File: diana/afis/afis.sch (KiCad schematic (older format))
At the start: 88 parts

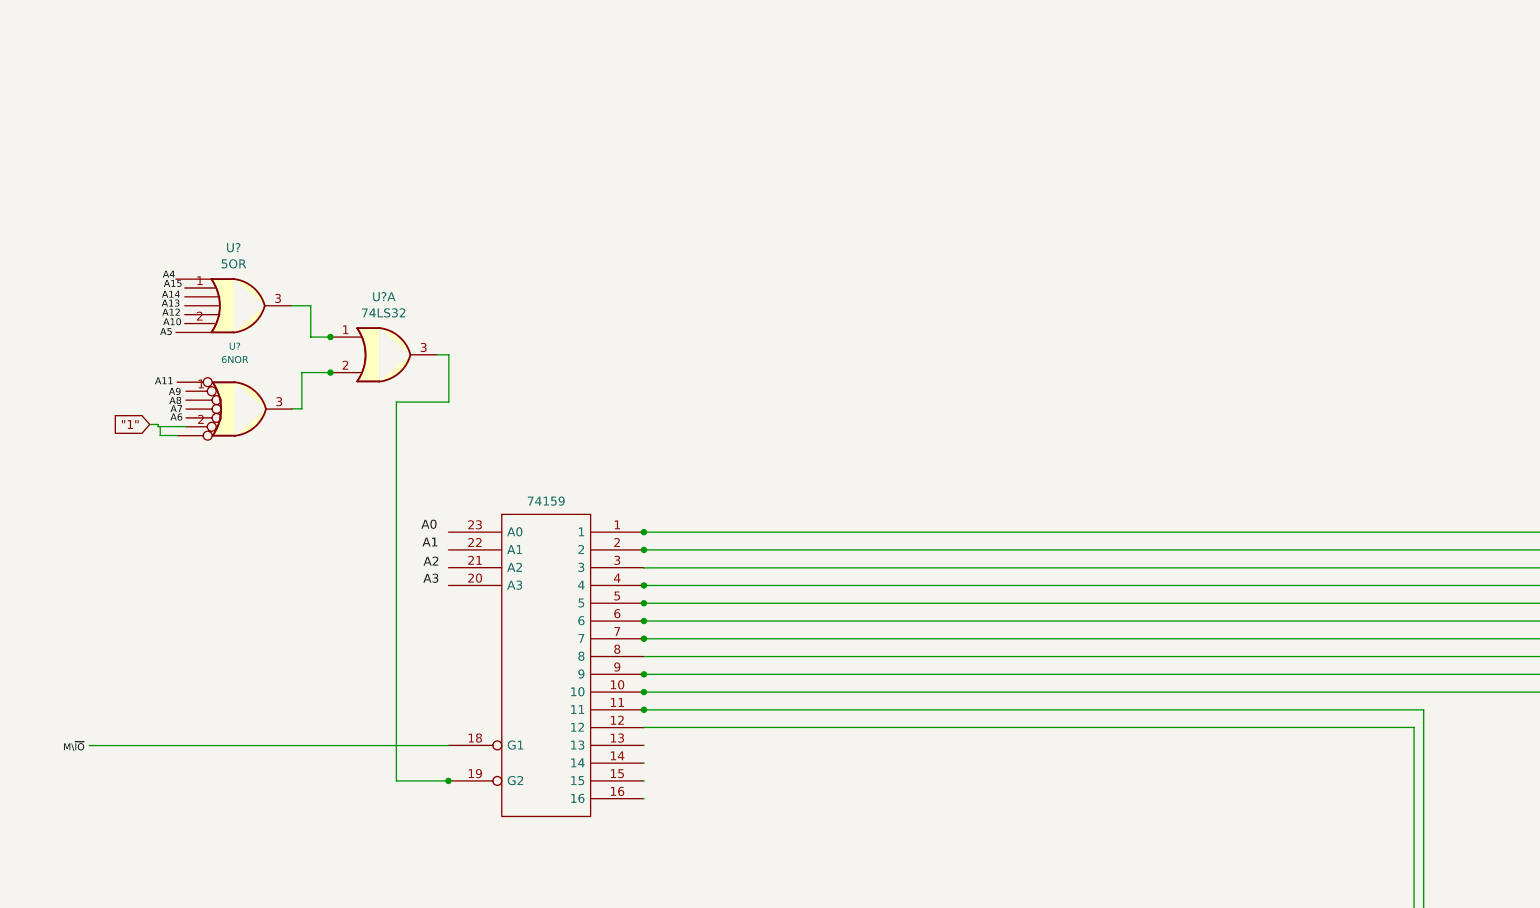
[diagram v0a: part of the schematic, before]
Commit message: c
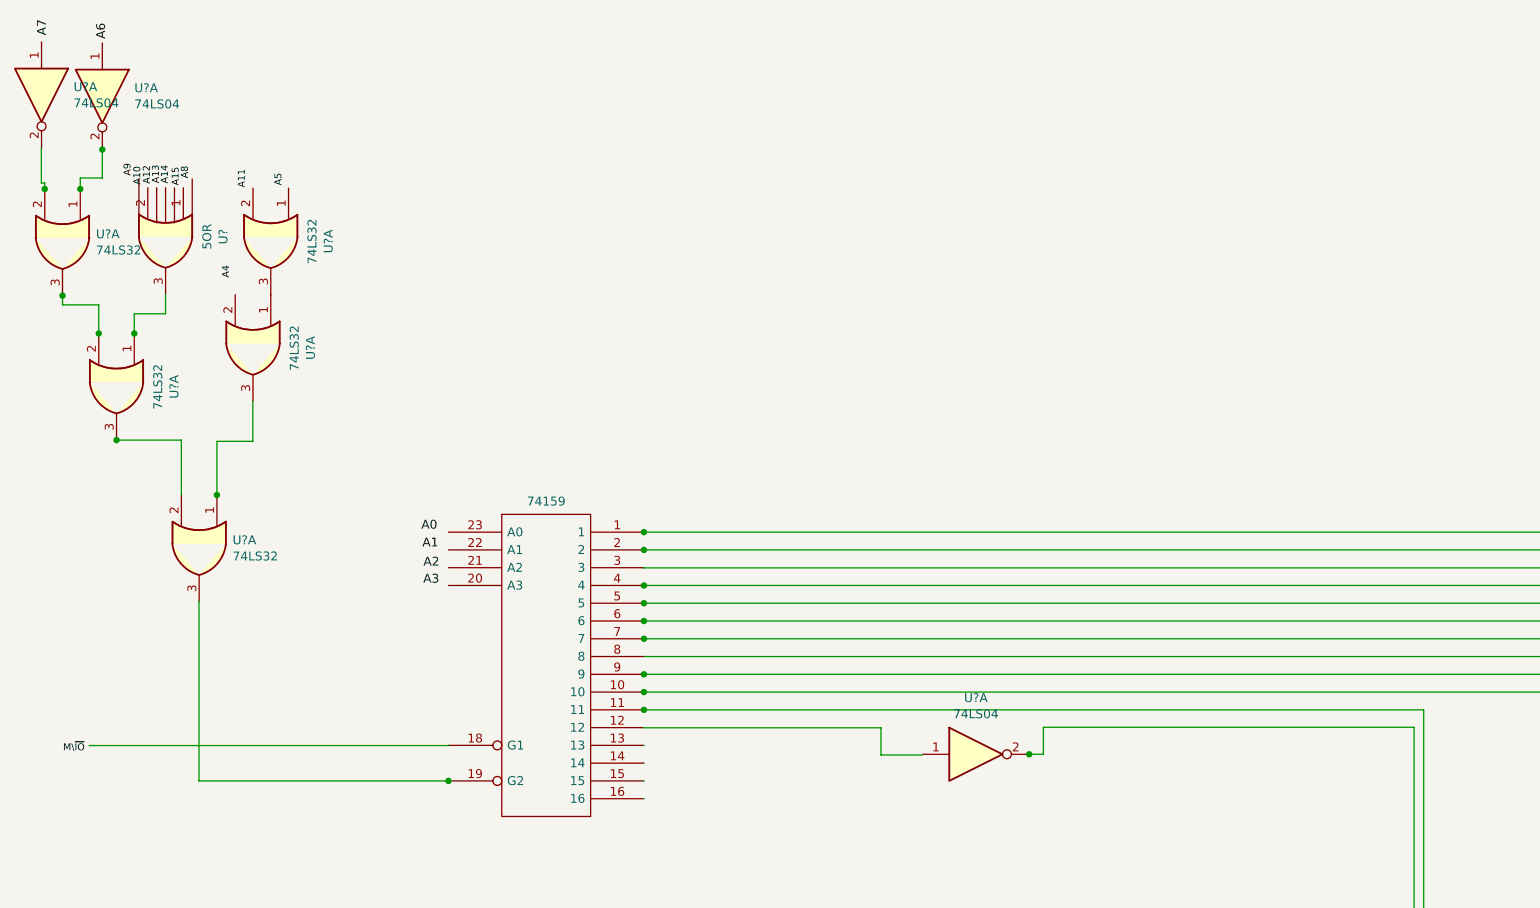
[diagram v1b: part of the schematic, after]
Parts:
- removed U?: 6NOR, symbol afis-rescue:6NOR-PMD-pmd-rescue
- added U? (x4): 74LS32, symbol 74xx:74LS32
- added U? (x3): 74LS04, symbol 74xx:74LS04
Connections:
- net labels removed: "1"
- wire segments 358 -> 373
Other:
- moved on the sheet: U?, U?A
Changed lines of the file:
@@
 L afis-rescue:5OR-PMD-pmd-rescue U?
 U 1 1 5DE3AD6A
-P 1860 5302
-F 0 "U?" H 1835 5877 50  0000 C CNN
-F 1 "5OR" H 1835 5786 50  0000 C CNN
-F 2 "" H 1810 5352 50  0001 C CNN
-F 3 "" H 1810 5352 50  0001 C CNN
-	1    1860 5302
-	1    0    0    -1
-$EndComp
-Text Label 1442 4962 0    39   ~ 0
+P 1202 4688
+F 0 "U?" H 1177 5263 50  0000 C CNN
+F 1 "5OR" H 1177 5172 50  0000 C CNN
+F 2 "" H 1152 4738 50  0001 C CNN
+F 3 "" H 1152 4738 50  0001 C CNN
+	1    1202 4688
+	0    1    1    0
+$EndComp
+Text Label 1542 4270 3    39   ~ 0
 A15
-Text Label 1431 5023 0    39   ~ 0
+Text Label 1481 4259 3    39   ~ 0
 A14
-Text Label 1430 5073 0    39   ~ 0
+Text Label 1431 4258 3    39   ~ 0
 A13
-Text Label 1433 5124 0    39   ~ 0
+Text Label 1380 4261 3    39   ~ 0
 A12
-Text Label 1438 5178 0    39   ~ 0
+Text Label 1326 4266 3    39   ~ 0
 A10
-Text Label 1421 5233 0    39   ~ 0
-A5
-Text Label 1436 4910 0    39   ~ 0
-A4
-Text Label 1392 5510 0    39   ~ 0
-A11
-Text Label 1470 5570 0    39   ~ 0
+Text Label 1271 4249 3    39   ~ 0
 A9
-Text Label 1473 5621 0    39   ~ 0
+Text Label 1594 4264 3    39   ~ 0
 A8
-Text Label 1479 5667 0    39   ~ 0
-A7
-Text Label 1479 5714 0    39   ~ 0
-A6
-$Comp
-L afis-rescue:6NOR-PMD-pmd-rescue U?
-U 1 1 5DF9DAE4
-P 1842 5957
-F 0 "U?" H 1842 6633 39  0000 C CNN
-F 1 "6NOR" H 1842 6558 39  0000 C CNN
-F 2 "" H 1842 5957 39  0001 C CNN
-F 3 "" H 1842 5957 39  0001 C CNN
-	1    1842 5957
-	1    0    0    -1
-$EndComp
 $Comp
 L 74xx:74LS32 U?
 U 1 1 5E02C74C
-P 2680 5328
-F 0 "U?" H 2680 5653 50  0000 C CNN
-F 1 "74LS32" H 2680 5562 50  0000 C CNN
-F 2 "" H 2680 5328 50  0001 C CNN
-F 3 "http://www.ti.com/lit/gpn/sn74LS32" H 2680 5328 50  0001 C CNN
-	1    2680 5328
-	1    0    0    -1
-$EndComp
-Wire Wire Line
-	2160 5052 2269 5052
-Wire Wire Line
-	2269 5052 2269 5228
-Wire Wire Line
-	2269 5228 2380 5228
-Connection ~ 2380 5228
-Wire Wire Line
-	2380 5228 2382 5228
-Wire Wire Line
-	2381 5428 2380 5428
-Wire Wire Line
-	2219 5428 2219 5632
-Wire Wire Line
-	2219 5632 2166 5632
-Connection ~ 2380 5428
-Wire Wire Line
-	2380 5428 2219 5428
-Wire Wire Line
-	2980 5328 3046 5328
-Wire Wire Line
-	3046 5328 3046 5594
-Wire Wire Line
-	3046 5594 2751 5594
-Wire Wire Line
-	2751 5594 2751 7726
-Wire Wire Line
-	2751 7726 3044 7726
+P 1176 5508
+F 0 "U?" H 1176 5833 50  0000 C CNN
+F 1 "74LS32" H 1176 5742 50  0000 C CNN
+F 2 "" H 1176 5508 50  0001 C CNN
+F 3 "http://www.ti.com/lit/gpn/sn74LS32" H 1176 5508 50  0001 C CNN
+	1    1176 5508
+	0    1    1    0
+$EndComp
+Wire Wire Line
+	1452 4988 1452 5097
+Wire Wire Line
+	1452 5097 1276 5097
+Wire Wire Line
+	1276 5097 1276 5208
+Connection ~ 1276 5208
+Wire Wire Line
+	1276 5208 1276 5210
+Wire Wire Line
+	1076 5209 1076 5208
+Wire Wire Line
+	1076 5047 872  5047
+Wire Wire Line
+	872  5047 872  4995
+Connection ~ 1076 5208
+Wire Wire Line
+	1076 5208 1076 5047
 Connection ~ 3044 7726
 Wire Wire Line
 	3044 7726 3047 7726
-Text GLabel 1363 5720 0    50   Input ~ 0
-"1"
-Wire Wire Line
-	1364 5720 1410 5720
-Wire Wire Line
-	1410 5720 1410 5732
-Wire Wire Line
-	1410 5732 1569 5732
-Wire Wire Line
-	1422 5731 1422 5782
-Wire Wire Line
-	1422 5782 1518 5782
 Wire Wire Line
 	10014 8061 10538 8061
@@
 Wire Wire Line
 	8706 11736 8710 11736
-Wire Wire Line
-	4142 7425 8478 7425
 Wire Wire Line
 	8478 7425 8478 12120
@@
 	1    0    0    -1
 $EndComp
+$Comp
+L 74xx:74LS32 U?
+U 1 1 5C8F4EE7
+P 2044 4690
+F 0 "U?" H 2044 5015 50  0000 C CNN
+F 1 "74LS32" H 2044 4924 50  0000 C CNN
+F 2 "" H 2044 4690 50  0001 C CNN
+F 3 "http://www.ti.com/lit/gpn/sn74LS32" H 2044 4690 50  0001 C CNN
+	1    2044 4690
+	0    1    1    0
+$EndComp
+Text Label 1914 4282 3    39   ~ 0
+A11
+Text Label 2120 4304 3    39   ~ 0
+A5
+$Comp
+L 74xx:74LS32 U?
+U 1 1 5C942EF5
+P 1944 5290
+F 0 "U?" H 1944 5615 50  0000 C CNN
+F 1 "74LS32" H 1944 5524 50  0000 C CNN
+F 2 "" H 1944 5290 50  0001 C CNN
+F 3 "http://www.ti.com/lit/gpn/sn74LS32" H 1944 5290 50  0001 C CNN
+	1    1944 5290
+	0    1    1    0
+$EndComp
+Text Label 1825 4823 3    39   ~ 0
+A4
+$Comp
+L 74xx:74LS32 U?
+U 1 1 5C9B81C8
+P 1641 6417
+F 0 "U?" V 1595 6605 50  0000 L CNN
+F 1 "74LS32" V 1686 6605 50  0000 L CNN
+F 2 "" H 1641 6417 50  0001 C CNN
+F 3 "http://www.ti.com/lit/gpn/sn74LS32" H 1641 6417 50  0001 C CNN
+	1    1641 6417
+	0    1    1    0
+$EndComp
+Wire Wire Line
+	1175 5808 1176 5808
+Wire Wire Line
+	1541 5808 1541 6117
+Connection ~ 1176 5808
+Wire Wire Line
+	1176 5808 1541 5808
+Wire Wire Line
+	1741 6118 1741 6117
+Wire Wire Line
+	1741 5815 1943 5815
+Wire Wire Line
+	1943 5815 1943 5590
+Connection ~ 1741 6117
+Wire Wire Line
+	1741 6117 1741 5815
+$Comp
+L 74xx:74LS32 U?
+U 1 1 5CE479B7
+P 872 4695
+F 0 "U?" V 826 4883 50  0000 L CNN
+F 1 "74LS32" V 917 4883 50  0000 L CNN
+F 2 "" H 872 4695 50  0001 C CNN
+F 3 "http://www.ti.com/lit/gpn/sn74LS32" H 872 4695 50  0001 C CNN
+	1    872  4695
+	0    1    1    0
+$EndComp
+Connection ~ 872  4995
+Wire Wire Line
+	872  4995 872  4994
+Text Label 798  3530 1    50   ~ 0
+A7
+Text Label 1131 3550 1    50   ~ 0
+A6
+$Comp
+L 74xx:74LS04 U?
+U 1 1 5CE96FE8
+P 754 3867
+F 0 "U?" V 708 4047 50  0000 L CNN
+F 1 "74LS04" V 799 4047 50  0000 L CNN
+F 2 "" H 754 3867 50  0001 C CNN
+F 3 "http://www.ti.com/lit/gpn/sn74LS04" H 754 3867 50  0001 C CNN
+	1    754  3867
+	0    1    1    0
+$EndComp
+$Comp
+L 74xx:74LS04 U?
+U 1 1 5CE97134
+P 1096 3873
+F 0 "U?" V 1050 4053 50  0000 L CNN
+F 1 "74LS04" V 1141 4053 50  0000 L CNN
+F 2 "" H 1096 3873 50  0001 C CNN
+F 3 "http://www.ti.com/lit/gpn/sn74LS04" H 1096 3873 50  0001 C CNN
+	1    1096 3873
+	0    1    1    0
+$EndComp
+Wire Wire Line
+	753  4164 753  4361
+Wire Wire Line
+	753  4361 772  4361
+Wire Wire Line
+	772  4361 772  4395
+Connection ~ 772  4395
+Wire Wire Line
+	772  4395 772  4397
+Wire Wire Line
+	1096 4171 1096 4173
+Wire Wire Line
+	1096 4333 972  4333
+Wire Wire Line
+	972  4333 972  4395
+Connection ~ 1096 4173
+Wire Wire Line
+	1096 4173 1096 4333
+Connection ~ 972  4395
+Wire Wire Line
+	972  4395 972  4396
+Wire Wire Line
+	1640 6714 1640 7726
+Wire Wire Line
+	1640 7726 3044 7726
+$Comp
+L 74xx:74LS04 U?
+U 1 1 5CF9A114
+P 6012 7576
+F 0 "U?" H 6012 7893 50  0000 C CNN
+F 1 "74LS04" H 6012 7802 50  0000 C CNN
+F 2 "" H 6012 7576 50  0001 C CNN
+F 3 "http://www.ti.com/lit/gpn/sn74LS04" H 6012 7576 50  0001 C CNN
+	1    6012 7576
+	1    0    0    -1
+$EndComp
+Wire Wire Line
+	4142 7427 5478 7427
+Wire Wire Line
+	5478 7427 5478 7580
+Wire Wire Line
+	5478 7580 5712 7580
+Wire Wire Line
+	6310 7576 6312 7576
+Wire Wire Line
+	6392 7576 6392 7424
+Wire Wire Line
+	6392 7424 8478 7424
+Connection ~ 6312 7576
+Wire Wire Line
+	6312 7576 6392 7576
 $EndSCHEMATC
